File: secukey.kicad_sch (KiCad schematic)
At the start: 44 parts, among them SW4 TS-1185-W-4P-H1.8-160, SW5 TS-1185-W-4P-H1.8-160, SW6 TS-1185-W-4P-H1.8-160, U2 RP2350A, U3 NCP1117-3.3_SOT223, U4 W25Q128JVS, U5 ABM8-272-T3_C20625731, U6 SM03B-SRSS-TB, U7 ATECC608A-MAHDA-T

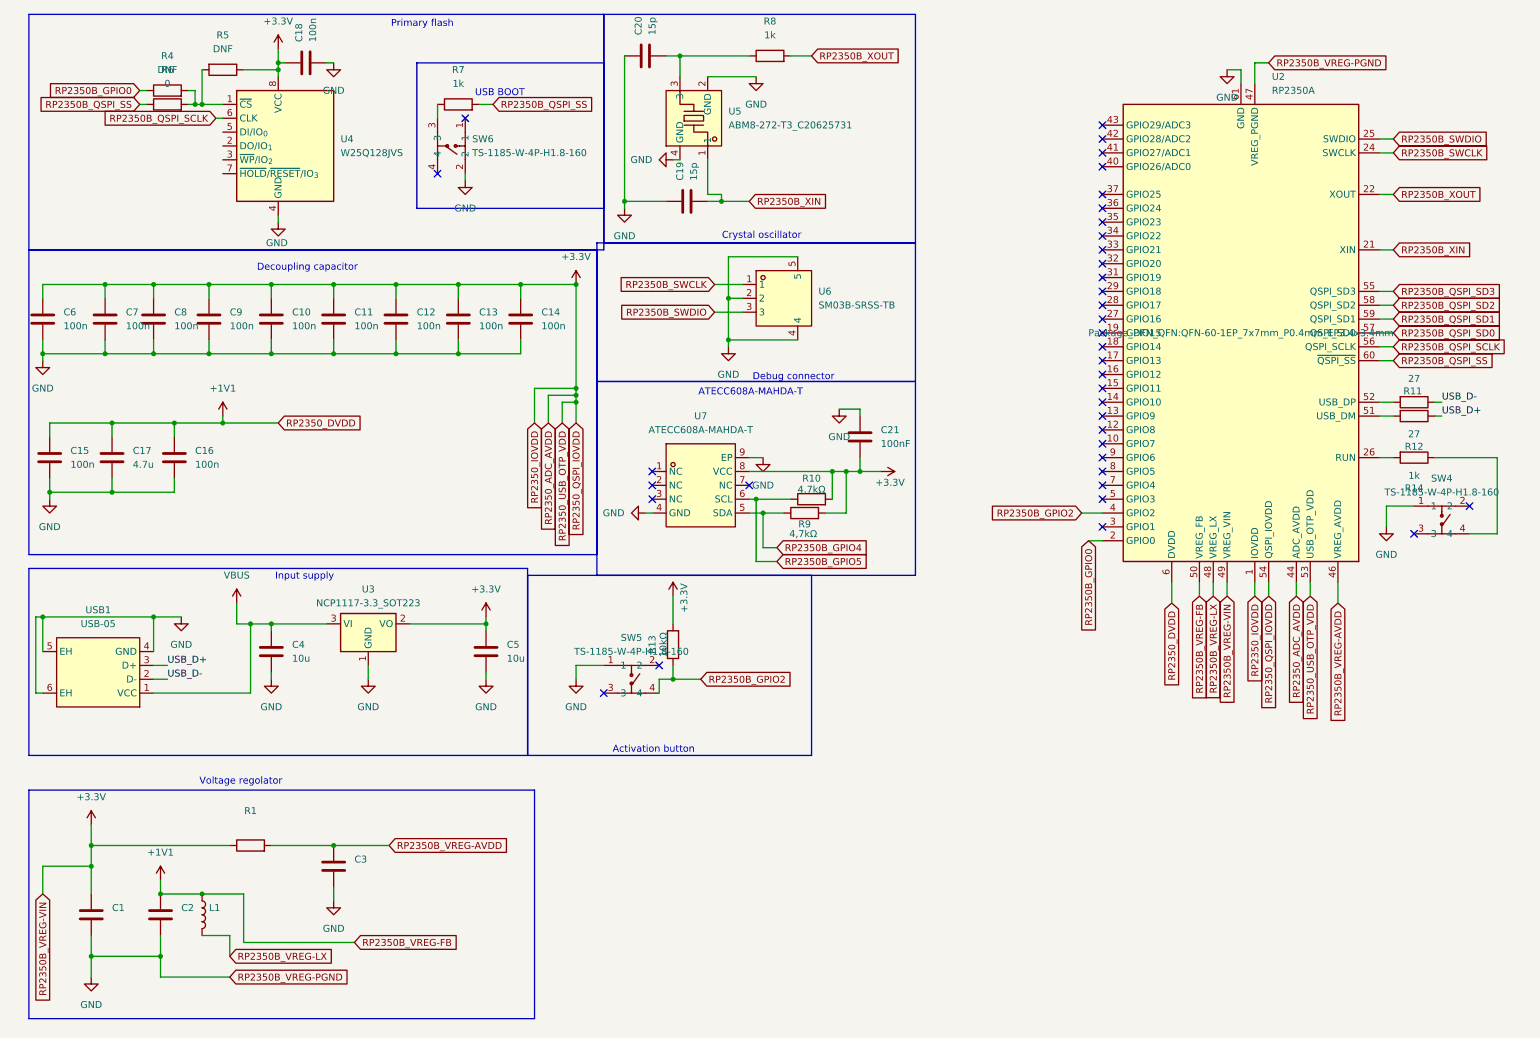
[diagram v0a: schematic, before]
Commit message: adding ref
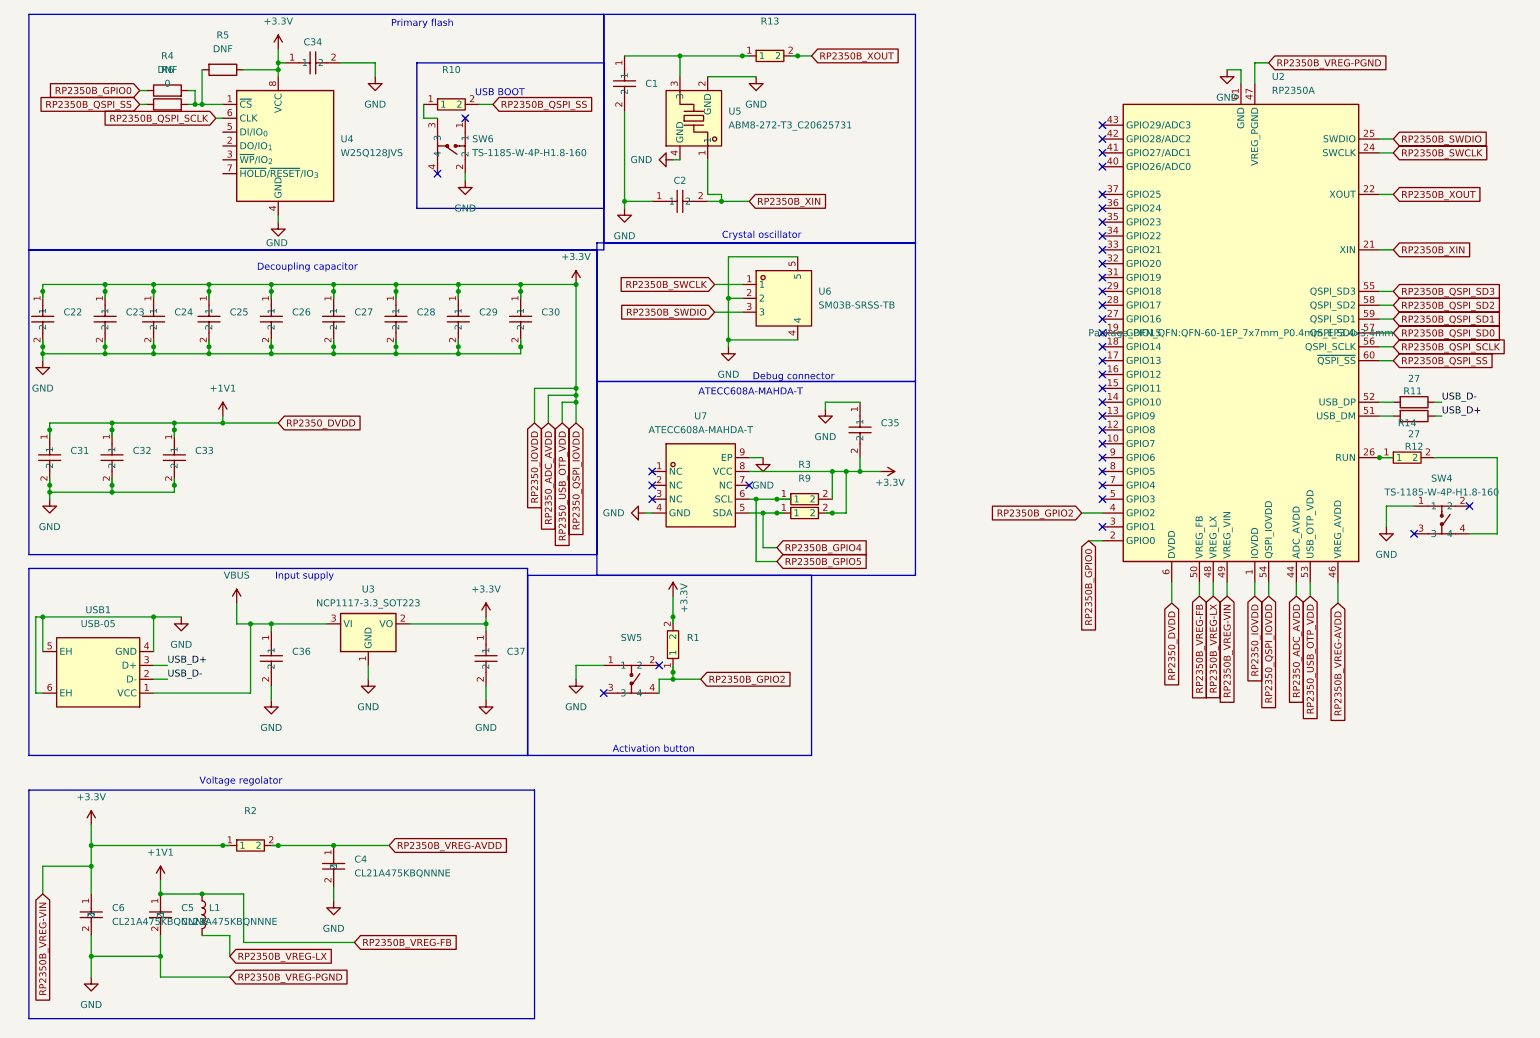
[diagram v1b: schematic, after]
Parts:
- removed C1, C17, C2, C3: 4.7u, Capacitor_SMD:C_0402_1005Metric, symbol Device:C
- removed C10, C11, C12, C13, C14, C15, C16, C18, C6, C7, C8, C9: 100n, Capacitor_SMD:C_0402_1005Metric, symbol Device:C
- removed C19, C20: 15p, Capacitor_SMD:C_0402_1005Metric, symbol Device:C
- removed C21: 100nF, Capacitor_SMD:C_0402_1005Metric, symbol Device:C
- removed C4, C5: 10u, Capacitor_SMD:C_0402_1005Metric, symbol Device:C
- removed R1: 33Ω, Resistor_SMD:R_0402_1005Metric, symbol Device:R
- removed R10, R9: 4,7kΩ, Resistor_SMD:R_0402_1005Metric, symbol Device:R
- removed R13: 10kΩ, Resistor_SMD:R_0402_1005Metric, symbol Device:R
- removed R14, R7, R8: 1k, Resistor_SMD:R_0402_1005Metric, symbol Device:R
- added C1, C2: FCC0805N150J500BT, EasyEDA:C0805, symbol EasyEDA:FCC0805N150J500BT
- added C22, C23, C24, C25, C26, C27, C28, C29, C30, C31, C32, C33, C34, C35, C36, C37: CC0402KRX7R5BB104, EasyEDA:C0402, symbol EasyEDA:CC0402KRX7R5BB104
- added C4, C5, C6: CL21A475KBQNNNE, EasyEDA:C0805, symbol EasyEDA:CL21A475KBQNNNE
- added R1: RC0805JR-0710KL, EasyEDA:R0805, symbol EasyEDA:RC0805JR-0710KL
- added R10, R13, R14: RC0805JR-071KL, EasyEDA:R0805, symbol EasyEDA:RC0805JR-071KL
- added R2: 0805W8J0330T5E, EasyEDA:R0805, symbol EasyEDA:0805W8J0330T5E
- added R3, R9: 0805W8F4701T5E, EasyEDA:R0805, symbol EasyEDA:0805W8F4701T5E
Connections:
- net +1V1: now also C31.1, C32.1, C33.1, C5.1
- net +3.3V: now also C22.1, C23.1, C24.1, C25.1, C26.1, C27.1, C28.1, C29.1, C30.1, C34.1, C35.2, C37.1, C6.1, R1.2, R2.1, R3.2, R9.2
- net GND: now also C1.2, C2.1, C22.2, C23.2, C24.2, C25.2, C26.2, C27.2, C28.2, C29.2, C30.2, C31.2, C32.2, C33.2, C34.2, C35.1, C36.2, C37.2, C4.2, C5.2, C6.2
- net RP2350B_GPIO2: now also R1.1
- net RP2350B_GPIO4: now also R9.1
- net RP2350B_GPIO5: now also R3.1
- net RP2350B_QSPI_SS: now also R10.2
- net RP2350B_VREG-AVDD: now also C4.1, R2.2
- net RP2350B_XIN: now also C2.2
- net RP2350B_XOUT: now also R13.2
- net VBUS: now also C36.1
- net at SW4.4: now also R14.2
- net at U2.26 (RUN): now also R14.1
- net at SW6.3: now also R10.1
- net at U5.3: now also C1.1, R13.1

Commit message: adding made placement
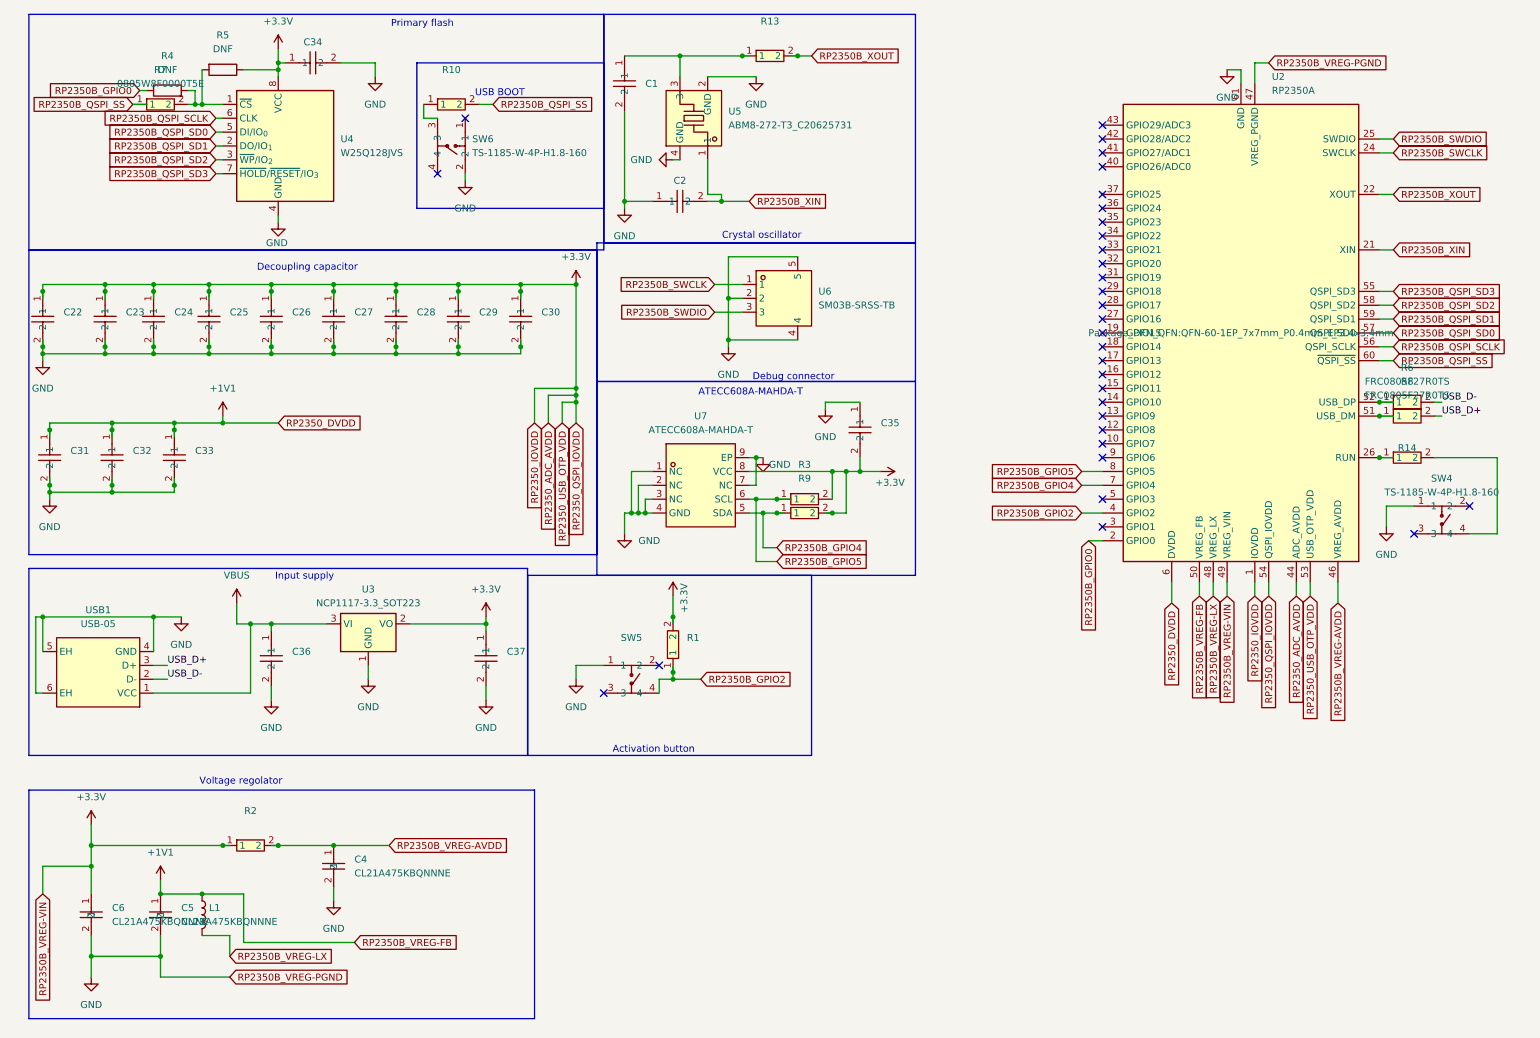
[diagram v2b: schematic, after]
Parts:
- removed R11, R12: 27, Resistor_SMD:R_0402_1005Metric, symbol Device:R
- removed R6: 0, Resistor_SMD:R_0402_1005Metric, symbol Device:R
- added R6, R8: FRC0805F27R0TS, EasyEDA:R0805, symbol EasyEDA:FRC0805F27R0TS
- added R7: 0805W8F0000T5E, EasyEDA:R0805, symbol EasyEDA:0805W8F0000T5E
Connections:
- net GND: now also U7.1 (NC), U7.2 (NC), U7.3 (NC), U7.7 (NC)
- net RP2350B_GPIO4: now also U2.7 (GPIO4)
- net RP2350B_GPIO5: now also U2.8 (GPIO5)
- net RP2350B_QSPI_SD0: now also U4.5 (DI/IO_{0})
- net RP2350B_QSPI_SD1: now also U4.2 (DO/IO_{1})
- net RP2350B_QSPI_SD2: now also U4.3 (~{WP}/IO_{2})
- net RP2350B_QSPI_SD3: now also U4.7 (~{HOLD}/~{RESET}/IO_{3})
- net RP2350B_QSPI_SS: now also R7.1
- net USB_D+: now also R8.2
- net USB_D-: now also R6.2
- net at U2.51 (USB_DM): now also R8.1
- net at R4.2, R5.2, U4.1 (~{CS}): now also R7.2
- net at U2.52 (USB_DP): now also R6.1
- no-connect marks 38 -> 32
